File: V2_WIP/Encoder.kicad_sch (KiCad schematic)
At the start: 12 parts, among them SW701 RotaryEncoder

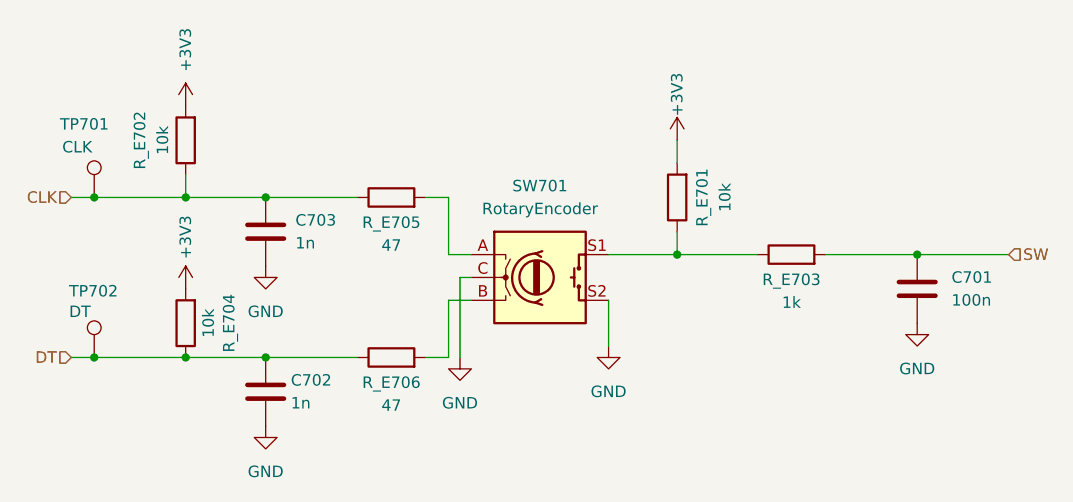
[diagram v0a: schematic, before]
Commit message: updated most datashets
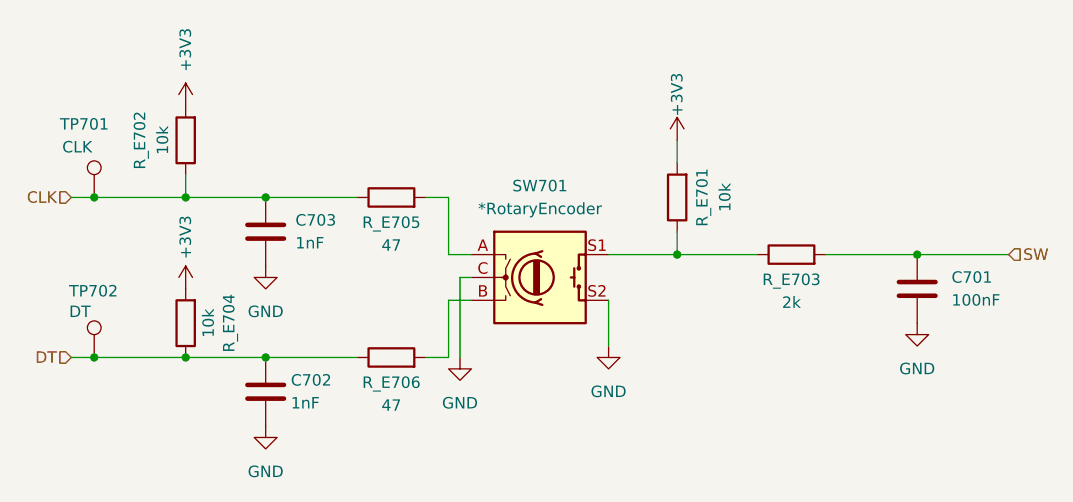
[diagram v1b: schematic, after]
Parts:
- C701: value 100n -> 100nF
- C702, C703: value 1n -> 1nF
- R_E703: value 1k -> 2k
- SW701: value RotaryEncoder -> *RotaryEncoder
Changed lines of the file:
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@@
 			)
 		)
-		(property "Datasheet" "~"
+		(property "Datasheet" "https://cz.mouser.com/ProductDetail/SEI-Stackpole/RNCE0603BTE10K0?qs=sGAEpiMZZMtlubZbdhIBIGfmJML7fLMVDBbNntjsT8g%3D"
 			(at 161.29 80.01 0)
 			(effects
@@
 			)
 		)
+		(property "Purchase-URL" ""
+			(at 161.29 80.01 0)
+			(effects
+				(font
+					(size 1.27 1.27)
+				)
+				(hide yes)
+			)
+		)
 		(pin "1"
 		)
@@
 			)
 		)
-		(property "Value" "1k"
+		(property "Value" "2k"
 			(at 173.99 91.694 90)
 			(effects
@@
 			)
 		)
-		(property "Datasheet" "~"
+		(property "Datasheet" "https://cz.mouser.com/ProductDetail/SEI-Stackpole/RNCE0603BTE2K00?qs=sGAEpiMZZMtlubZbdhIBIGfmJML7fLMVr3bVQ0UuJPQ%3D"
 			(at 173.99 86.36 0)
 			(effects
@@
 			)
 		)
+		(property "Purchase-URL" ""
+			(at 173.99 86.36 0)
+			(effects
+				(font
+					(size 1.27 1.27)
+				)
+				(hide yes)
+			)
+		)
 		(pin "1"
 		)
@@
 			)
 		)
+		(property "Purchase-URL" ""
+			(at 96.52 80.01 0)
+			(effects
+				(font
+					(size 1.27 1.27)
+				)
+				(hide yes)
+			)
+		)
 		(pin "1"
 		)
@@
 			)
 		)
-		(property "Value" "1n"
+		(property "Value" "1nF"
 			(at 118.364 102.87 0)
 			(effects
@@
 			)
 		)
-		(property "Datasheet" "~"
+		(property "Datasheet" "https://cz.mouser.com/ProductDetail/KYOCERA-AVX/06031A102JAT2A?qs=%252BdQmOuGyFcGHJqs3Zmdykg%3D%3D"
 			(at 115.57 101.6 0)
 			(effects
@@
 		)
 		(property "Description" "Unpolarized capacitor"
+			(at 115.57 101.6 0)
+			(effects
+				(font
+					(size 1.27 1.27)
+				)
+				(hide yes)
+			)
+		)
+		(property "Purchase-URL" ""
 			(at 115.57 101.6 0)
 			(effects
@@
 			)
 		)
-		(property "Value" "RotaryEncoder"
+		(property "Value" "*RotaryEncoder"
 			(at 146.05 81.28 0)
 			(effects
@@
 			)
 		)
+		(property "Purchase-URL" ""
+			(at 146.05 88.9 0)
+			(effects
+				(font
+					(size 1.27 1.27)
+				)
+				(hide yes)
+			)
+		)
 		(pin "A"
 		)
@@
 			)
 		)
-		(property "Datasheet" "~"
+		(property "Datasheet" "https://cz.mouser.com/ProductDetail/Vishay-Beyschlag/MCT06030D4709BP500?qs=sGAEpiMZZMtlubZbdhIBIOF8iwLVxXp6Oa2rPEx3MVU%3D"
 			(at 129.54 80.01 0)
 			(effects
@@
 			)
 		)
+		(property "Purchase-URL" ""
+			(at 129.54 80.01 0)
+			(effects
+				(font
+					(size 1.27 1.27)
+				)
+				(hide yes)
+			)
+		)
 		(pin "1"
 		)
@@
 			)
 		)
+		(property "Purchase-URL" ""
+			(at 96.52 97.79 0)
+			(effects
+				(font
+					(size 1.27 1.27)
+				)
+				(hide yes)
+			)
+		)
 		(pin "1"
 		)
@@
 			)
 		)
-		(property "Datasheet" "~"
+		(property "Datasheet" "https://cz.mouser.com/ProductDetail/SEI-Stackpole/RNCE0603BTE10K0?qs=sGAEpiMZZMtlubZbdhIBIGfmJML7fLMVDBbNntjsT8g%3D"
 			(at 106.68 93.98 0)
 			(effects
@@
 			)
 		)
+		(property "Purchase-URL" ""
+			(at 106.68 93.98 0)
+			(effects
+				(font
+					(size 1.27 1.27)
+				)
+				(hide yes)
+			)
+		)
 		(pin "1"
 		)
@@
 			)
 		)
-		(property "Value" "1n"
+		(property "Value" "1nF"
 			(at 118.872 85.09 0)
 			(effects
@@
 			)
 		)
-		(property "Datasheet" "~"
+		(property "Datasheet" "https://cz.mouser.com/ProductDetail/KYOCERA-AVX/06031A102JAT2A?qs=%252BdQmOuGyFcGHJqs3Zmdykg%3D%3D"
 			(at 115.57 83.82 0)
 			(effects
@@
 		)
 		(property "Description" "Unpolarized capacitor"
+			(at 115.57 83.82 0)
+			(effects
+				(font
+					(size 1.27 1.27)
+				)
+				(hide yes)
+			)
+		)
+		(property "Purchase-URL" ""
 			(at 115.57 83.82 0)
 			(effects
@@
 			)
 		)
-		(property "Datasheet" "~"
+		(property "Datasheet" "https://cz.mouser.com/ProductDetail/SEI-Stackpole/RNCE0603BTE10K0?qs=sGAEpiMZZMtlubZbdhIBIGfmJML7fLMVDBbNntjsT8g%3D"
 			(at 106.68 73.66 0)
 			(effects
@@
 			)
 		)
+		(property "Purchase-URL" ""
+			(at 106.68 73.66 0)
+			(effects
+				(font
+					(size 1.27 1.27)
+				)
+				(hide yes)
+			)
+		)
 		(pin "1"
 		)
@@
 			)
 		)
-		(property "Datasheet" "~"
+		(property "Datasheet" "https://cz.mouser.com/ProductDetail/Vishay-Beyschlag/MCT06030D4709BP500?qs=sGAEpiMZZMtlubZbdhIBIOF8iwLVxXp6Oa2rPEx3MVU%3D"
 			(at 129.54 97.79 0)
 			(effects
@@
 		)
 		(property "Description" "Resistor"
+			(at 129.54 97.79 0)
+			(effects
+				(font
+					(size 1.27 1.27)
+				)
+				(hide yes)
+			)
+		)
+		(property "Purchase-URL" ""
 			(at 129.54 97.79 0)
 			(effects
@@
 			)
 		)
-		(property "Value" "100n"
+		(property "Value" "100nF"
 			(at 191.77 91.4399 0)
 			(effects
@@
 			)
 		)
-		(property "Datasheet" "~"
+		(property "Datasheet" "https://cz.mouser.com/ProductDetail/KYOCERA-AVX/0603ZG104ZAT2A?qs=XWDBCzcA0Tke70DI9cEVbA%3D%3D"
 			(at 187.96 90.17 0)
 			(effects
@@
 			(at 187.96 90.17 0)
 			(effects
+				(font
+					(size 1.27 1.27)
+				)
+				(hide yes)
+			)
+		)
+		(property "Purchase-URL" ""
+			(at 187.96 90.17 0)
+			(effects

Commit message: up to date i dont remember what changed
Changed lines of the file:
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@@
 (kicad_sch
-	(version 20231120)
+	(version 20250114)
 	(generator "eeschema")
-	(generator_version "8.0")
+	(generator_version "9.0")
 	(paper "A4")
 	(junction
@@
 		(shape input)
 		(at 93.98 97.79 180)
-		(fields_autoplaced yes)
 		(effects
 			(font
@@
 		(shape input)
 		(at 93.98 80.01 180)
-		(fields_autoplaced yes)
 		(effects
 			(font
@@
 		(shape input)
 		(at 198.12 86.36 0)
-		(fields_autoplaced yes)
 		(effects
 			(font
